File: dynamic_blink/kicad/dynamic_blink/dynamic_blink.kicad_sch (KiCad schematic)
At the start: 3 parts, among them SW1 Momentary Switch

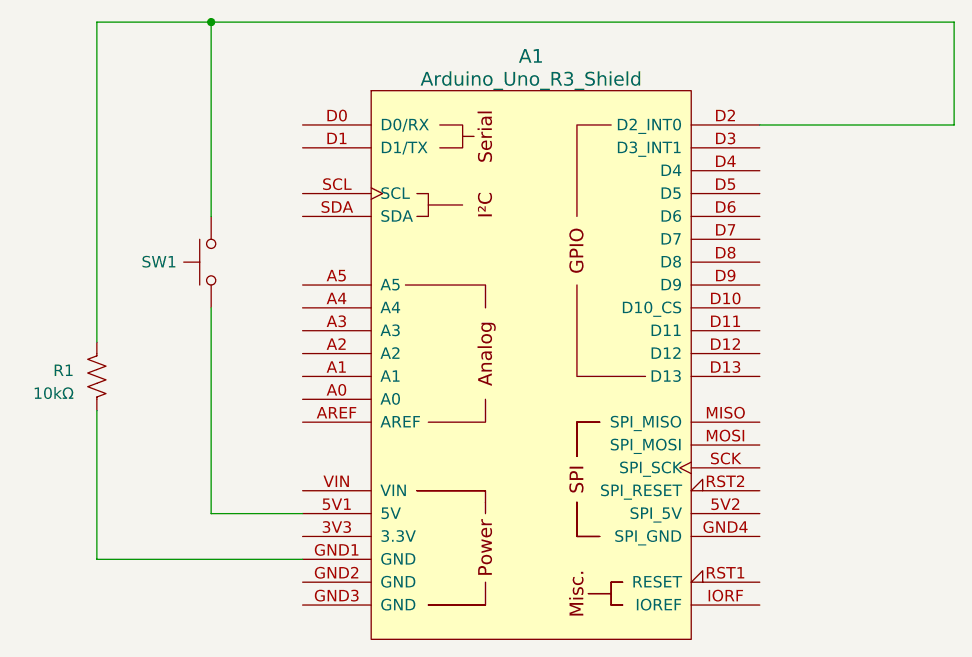
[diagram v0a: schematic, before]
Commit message: Use default Arduino UNO R3 symbol
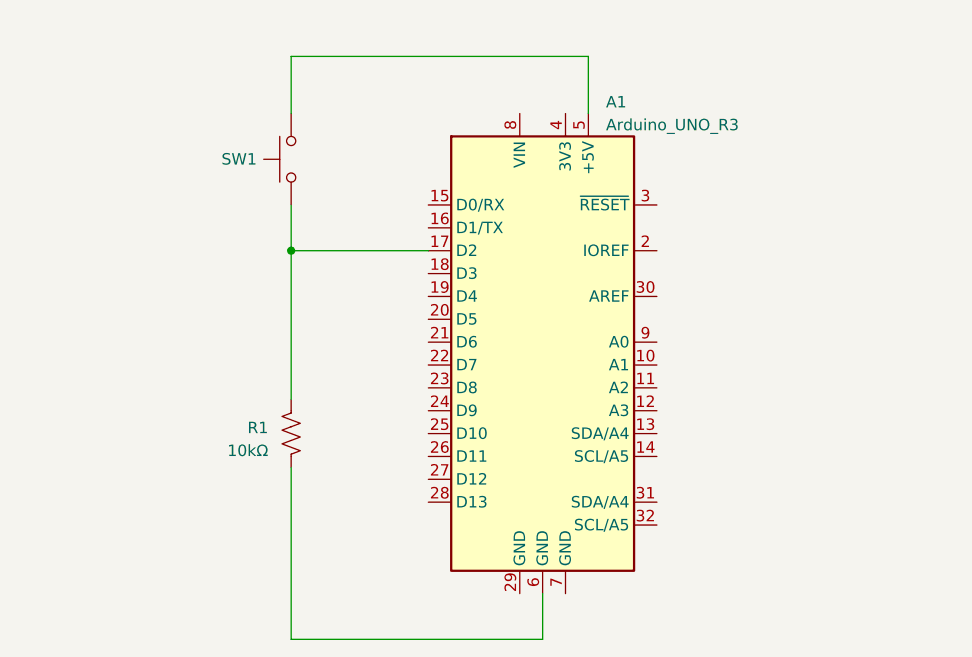
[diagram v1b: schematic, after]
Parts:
- removed A1: Arduino_Uno_R3_Shield, PCM_arduino-library:Arduino_Uno_R3_Shield, symbol PCM_arduino-library:Arduino_Uno_R3_Shield
- added A1: Arduino_UNO_R3, Module:Arduino_UNO_R3, symbol MCU_Module:Arduino_UNO_R3
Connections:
- net at R1.1: now also SW1.2, A1.17 (D2); no longer SW1.1
- net at R1.2: now also A1.6 (GND)
- new net: A1.5 (+5V), SW1.1
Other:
- moved on the sheet: R1, SW1
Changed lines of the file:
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@@
     (title "Dynamic Blink")
   )
-  (junction (at 66.04 24.13) (diameter 0) (color 0 0 0 0)
+  (junction (at 74.93 49.53) (diameter 0) (color 0 0 0 0)
   )
-  (wire (pts (xy 53.34 67.31) (xy 53.34 83.82))
+  (wire (pts (xy 74.93 92.71) (xy 102.87 92.71))
     (stroke (width 0) (type default))
   )
-  (wire (pts (xy 53.34 83.82) (xy 76.2 83.82))
+  (wire (pts (xy 107.95 34.29) (xy 107.95 27.94))
     (stroke (width 0) (type default))
   )
-  (wire (pts (xy 148.59 35.56) (xy 127 35.56))
+  (wire (pts (xy 102.87 92.71) (xy 102.87 87.63))
     (stroke (width 0) (type default))
   )
-  (wire (pts (xy 53.34 59.69) (xy 53.34 24.13))
+  (wire (pts (xy 74.93 73.66) (xy 74.93 92.71))
     (stroke (width 0) (type default))
   )
-  (wire (pts (xy 66.04 24.13) (xy 148.59 24.13))
+  (wire (pts (xy 107.95 27.94) (xy 74.93 27.94))
     (stroke (width 0) (type default))
   )
-  (wire (pts (xy 66.04 45.72) (xy 66.04 24.13))
+  (wire (pts (xy 74.93 49.53) (xy 90.17 49.53))
     (stroke (width 0) (type default))
   )
-  (wire (pts (xy 66.04 55.88) (xy 66.04 78.74))
+  (wire (pts (xy 74.93 44.45) (xy 74.93 49.53))
     (stroke (width 0) (type default))
   )
-  (wire (pts (xy 66.04 78.74) (xy 76.2 78.74))
+  (wire (pts (xy 74.93 49.53) (xy 74.93 66.04))
     (stroke (width 0) (type default))
   )
-  (wire (pts (xy 53.34 24.13) (xy 66.04 24.13))
+  (wire (pts (xy 74.93 27.94) (xy 74.93 34.29))
     (stroke (width 0) (type default))
   )
-  (wire (pts (xy 148.59 24.13) (xy 148.59 35.56))
-    (stroke (width 0) (type default))
-  )
-  (symbol (lib_id "Device:R_US") (at 53.34 63.5 0) (mirror y) (unit 1)
+  (symbol (lib_id "Device:R_US") (at 74.93 69.85 0) (mirror y) (unit 1)
     (in_bom yes) (on_board yes) (dnp no)
-    (property "Reference" "R1" (at 50.8 62.865 0)
+    (property "Reference" "R1" (at 72.39 69.215 0)
       (effects (font (size 1.27 1.27)) (justify left))
     )
-    (property "Value" "10kΩ" (at 50.8 65.405 0)
+    (property "Value" "10kΩ" (at 72.39 71.755 0)
       (effects (font (size 1.27 1.27)) (justify left))
     )
-    (property "Footprint" "" (at 52.324 63.754 90)
+    (property "Footprint" "" (at 73.914 70.104 90)
       (effects (font (size 1.27 1.27)) hide)
     )
-    (property "Datasheet" "~" (at 53.34 63.5 0)
+    (property "Datasheet" "~" (at 74.93 69.85 0)
       (effects (font (size 1.27 1.27)) hide)
     )
@@
     )
   )
-  (symbol (lib_id "PCM_arduino-library:Arduino_Uno_R3_Shield") (at 101.6 62.23 0) (unit 1)
-    (in_bom yes) (on_board yes) (dnp no) (fields_autoplaced)
-    (property "Reference" "A1" (at 101.6 27.94 0)
-      (effects (font (size 1.524 1.524)))
-    )
-    (property "Value" "Arduino_Uno_R3_Shield" (at 101.6 30.48 0)
-      (effects (font (size 1.524 1.524)))
-    )
-    (property "Footprint" "PCM_arduino-library:Arduino_Uno_R3_Shield" (at 101.6 100.33 0)
-      (effects (font (size 1.524 1.524)) hide)
-    )
-    (property "Datasheet" "https://docs.arduino.cc/hardware/uno-rev3" (at 101.6 96.52 0)
-      (effects (font (size 1.524 1.524)) hide)
-    )
-    (pin "3V3")
-    (pin "5V1")
-    (pin "5V2")
-    (pin "A0")
-    (pin "A1")
-    (pin "A2")
-    (pin "A3")
-    (pin "A4")
-    (pin "A5")
-    (pin "AREF")
-    (pin "D0")
-    (pin "D1")
-    (pin "D10")
-    (pin "D11")
-    (pin "D12")
-    (pin "D13")
-    (pin "D2")
-    (pin "D3")
-    (pin "D4")
-    (pin "D5")
-    (pin "D6")
-    (pin "D7")
-    (pin "D8")
-    (pin "D9")
-    (pin "GND1")
-    (pin "GND2")
-    (pin "GND3")
-    (pin "GND4")
-    (pin "IORF")
-    (pin "MISO")
-    (pin "MOSI")
-    (pin "RST1")
-    (pin "RST2")
-    (pin "SCK")
-    (pin "SCL")
-    (pin "SDA")
-    (pin "VIN")
-    (instances
-      (project "dynamic_blink"
-        (path "/062c7fc9-3203-4e28-9240-3193774e34ca"
-          (reference "A1") (unit 1)
-        )
-      )
-    )
-  )
-  (symbol (lib_id "Switch:SW_Push") (at 66.04 50.8 90) (mirror x) (unit 1)
+  (symbol (lib_id "Switch:SW_Push") (at 74.93 39.37 90) (mirror x) (unit 1)
     (in_bom yes) (on_board yes) (dnp no)
-    (property "Reference" "SW1" (at 62.23 50.8 90)
+    (property "Reference" "SW1" (at 71.12 39.37 90)
       (effects (font (size 1.27 1.27)) (justify left))
     )
-    (property "Value" "Momentary Switch" (at 62.23 52.705 90)
+    (property "Value" "Momentary Switch" (at 71.12 41.275 90)
       (effects (font (size 1.27 1.27)) (justify left) hide)
     )
-    (property "Footprint" "" (at 60.96 50.8 0)
+    (property "Footprint" "" (at 69.85 39.37 0)
       (effects (font (size 1.27 1.27)) hide)
     )
-    (property "Datasheet" "~" (at 60.96 50.8 0)
+    (property "Datasheet" "~" (at 69.85 39.37 0)
       (effects (font (size 1.27 1.27)) hide)
     )
@@
         )
       )
+    )
+  )
+  (symbol (lib_id "MCU_Module:Arduino_UNO_R3") (at 102.87 59.69 0) (unit 1)
+    (in_bom yes) (on_board yes) (dnp no) (fields_autoplaced)
+    (property "Reference" "A1" (at 109.9059 33.02 0)
+      (effects (font (size 1.27 1.27)) (justify left))
+    )
+    (property "Value" "Arduino_UNO_R3" (at 109.9059 35.56 0)
+      (effects (font (size 1.27 1.27)) (justify left))
+    )
+    (property "Footprint" "Module:Arduino_UNO_R3" (at 102.87 59.69 0)
+      (effects (font (size 1.27 1.27) italic) hide)
+    )
+    (property "Datasheet" "https://www.arduino.cc/en/Main/arduinoBoardUno" (at 102.87 59.69 0)
+      (effects (font (size 1.27 1.27)) hide)
+    )
+    (pin "1")
+    (pin "10")
+    (pin "11")
+    (pin "12")
+    (pin "13")
+    (pin "14")
+    (pin "15")
+    (pin "16")
+    (pin "17")
+    (pin "18")
+    (pin "19")
+    (pin "2")
+    (pin "20")
+    (pin "21")
+    (pin "22")
+    (pin "23")
+    (pin "24")
+    (pin "25")
+    (pin "26")
+    (pin "27")
+    (pin "28")
+    (pin "29")
+    (pin "3")
+    (pin "30")
+    (pin "31")
+    (pin "32")
+    (pin "4")
+    (pin "5")
+    (pin "6")
+    (pin "7")
+    (pin "8")
+    (pin "9")
+    (instances
+      (project "dynamic_blink"
+        (path "/062c7fc9-3203-4e28-9240-3193774e34ca"
+          (reference "A1") (unit 1)
+        )
+      )
